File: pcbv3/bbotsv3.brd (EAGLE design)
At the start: 60 x 60 mm, 15 parts

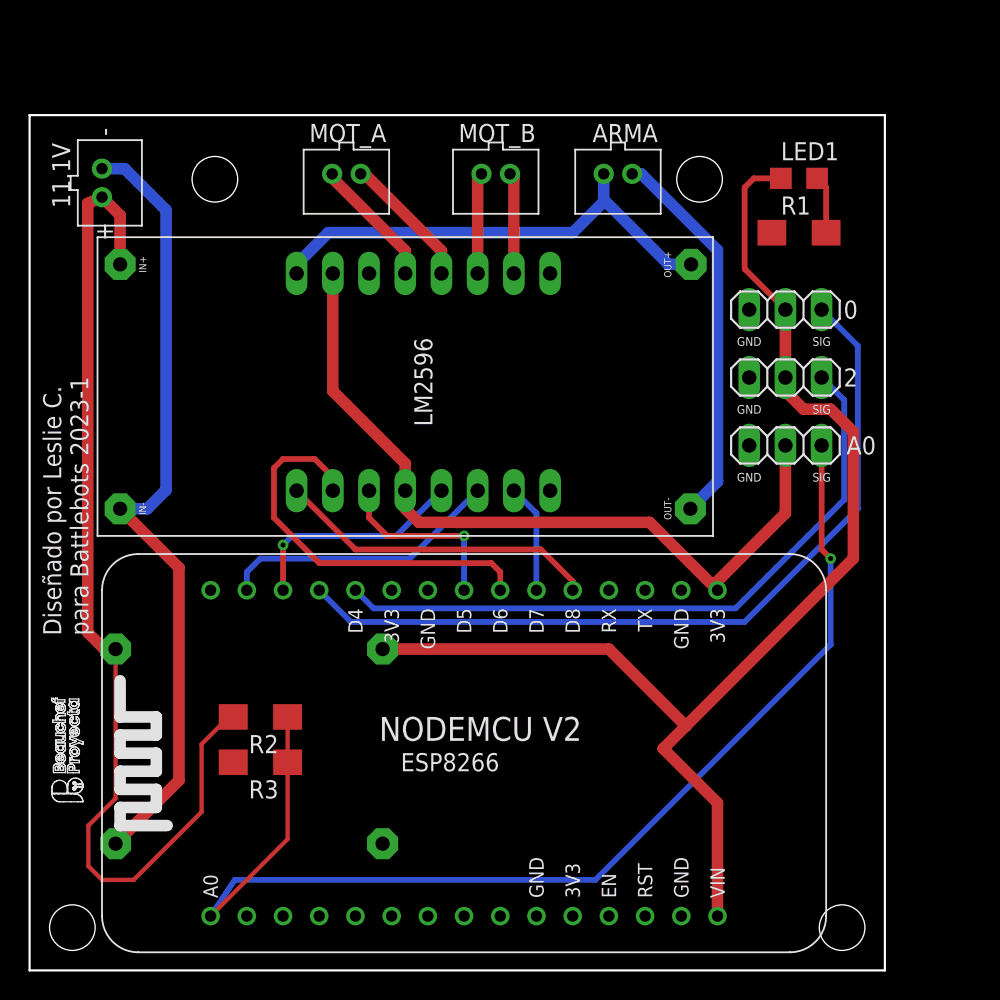
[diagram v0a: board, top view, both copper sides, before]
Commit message: finish pcb, waiting review
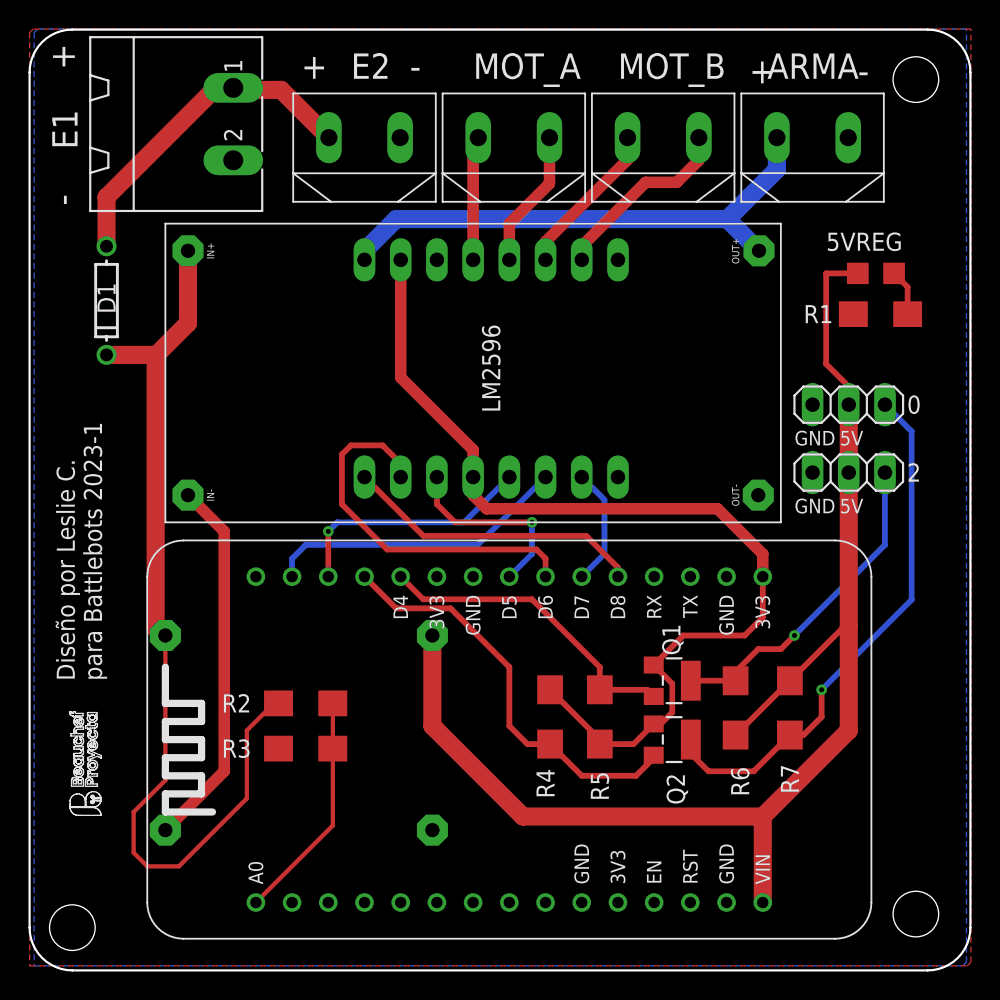
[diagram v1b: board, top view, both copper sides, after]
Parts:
- removed 11.1V: (no value), adafruit:JST-PH-2-THM
- removed A0: 3.3, my-library:1X03
- removed LED1: (no value), my-library:R0805
- removed MOT_A, MOT_B: (no value), my-library:JST_2PIN
- added 5VREG: (no value), my-library:R0805
- added ARMA1, ARMA2, ARMA3: TERMINAL_2P, KF301-2P-Terminal:KF301-2P
- added D1: (no value), adafruit:DO-1N4148
- added E1: MSTBA2, con-phoenix-508:MSTBA2
- added Q1, Q2: (no value), adafruit:SOT23-W
- added R4, R5, R6, R7: 10k, my-library:R1206
- ARMA: value (none) -> TERMINAL_2P; device my-library:JST_2PIN -> KF301-2P-Terminal:KF301-2P
- R1: value BB-R1205 -> 100
- R2: value BB-R1205 -> 10k
- R3: value BB-R1205 -> 1k
- moved ARMA 13.9 mm to (54.9, 58.4), turned to 0 degrees
- moved R1 8.08 mm to (59.7, 46.0)
- moved 2 8.01 mm to (57.5, 34.9)
- moved 0 8.01 mm to (57.5, 39.7)
- moved U$1 4.86 mm to (9.53, 52.4)
- moved U$2 4.86 mm to (32.4, 42.2)
- moved U$3 3.62 mm to (30.2, 25.1)
- moved R2 3.31 mm to (19.4, 18.7)
- moved R3 3.31 mm to (19.4, 15.6)
- moved NODE1 3.31 mm to (32.4, 16.2)
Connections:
- removed net N$16: MOT_B.2, U$2.BO1
- new net N$11: 2.S, Q1.3, R6.1
- new net N$19: NODE1.D4, Q1.2, R5.1
- new net N$2: ARMA3.1, D1.A, E1.1
- net 11.1: now also D1.C; no longer 11.1V.1
- net 3V3: now also NODE1.3V3@1, NODE1.3V3@3, Q1.1, Q2.1, R4.2, R5.2, U$2.STBY, U$2.VCC
- net 5V: now also 5VREG.1, R6.2, R7.2; no longer LED1.1
- net GND2: now also ARMA3.2, E1.2, U$2.GND2; no longer 11.1V.2, A0.GND
- net N$1: no longer A0.S
- net N$12: now also NODE1.D3, Q2.2, R4.1; no longer 2.S, NODE1.D4
- net N$13: now also ARMA1.2; no longer MOT_A.2
- net N$14: now also ARMA1.1; no longer MOT_A.1
- net N$15: now also ARMA2.2, U$2.BO1; no longer MOT_B.1, U$2.BO2
- net N$18: now also Q2.3, R7.1; no longer NODE1.D3
- net N$3: now also 5VREG.2; no longer LED1.2
- net N$6: now also ARMA2.1, U$2.BO2; no longer A0.P, NODE1.3V3@1, NODE1.3V3@3, U$2.STBY, U$2.VCC
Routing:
- net 3V3: track 0.00 -> 69.2 mm
- net N$1: track 82.1 -> 16.2 mm, vias 1 -> 0
- net GND2: track 83.3 -> 26.3 mm
- net N$6: track 55.0 -> 11.0 mm
- net N$2: track 0.00 -> 23.7 mm
- net N$11: track 0.00 -> 23.0 mm, vias 0 -> 1
- net N$19: track 0.00 -> 22.2 mm
- net N$18: track 57.0 -> 37.6 mm, vias 0 -> 1
- net N$12: track 47.2 -> 29.2 mm
- net 11.1: track 73.0 -> 65.8 mm
- net N$16: track 7.10 -> 0.00 mm
- net N$15: track 7.10 -> 13.3 mm
- net 5V: track 88.8 -> 92.8 mm
- net 12V: track 34.0 -> 37.3 mm
- net N$9: track 15.9 -> 17.5 mm
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- added copper zone on layer 1, net GND2
- added copper zone on layer 16, net GND2
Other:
- board size 60 x 60 mm -> 66 x 66 mm
- board text added: "+"
- board text added: "-"
- board text added: "5V"
- board text added: "ARMA"
- board text added: "Diseño por Leslie C. para Battlebots 2023-1"
- board text added: "E2"
- board text added: "GND"
- board text added: "MOT_A"
- board text added: "MOT_B"
- board text removed: "Diseñado por Leslie C. para Battlebots 2023-1"
